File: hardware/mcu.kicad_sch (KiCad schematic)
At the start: 36 parts, among them U1 74LVC125, U2 STM32F407VETx, U3 24LC64, U7 74LVC125, X1 12MHz

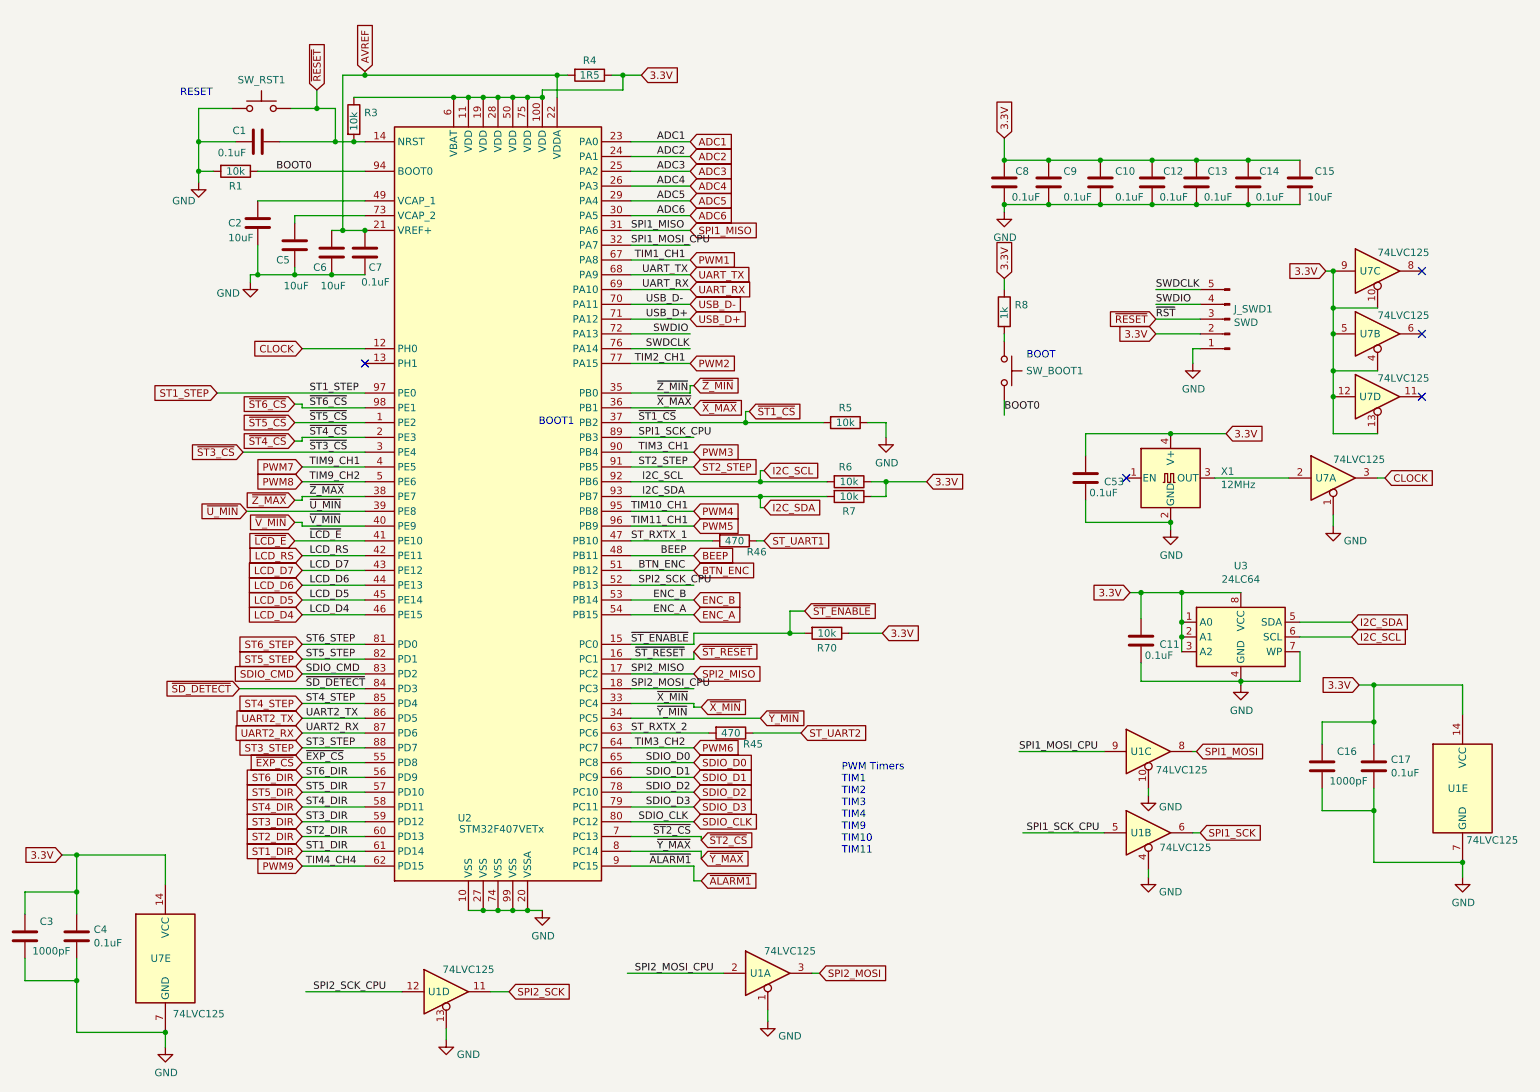
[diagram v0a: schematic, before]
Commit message: Update PrntrBoard fabrication files.
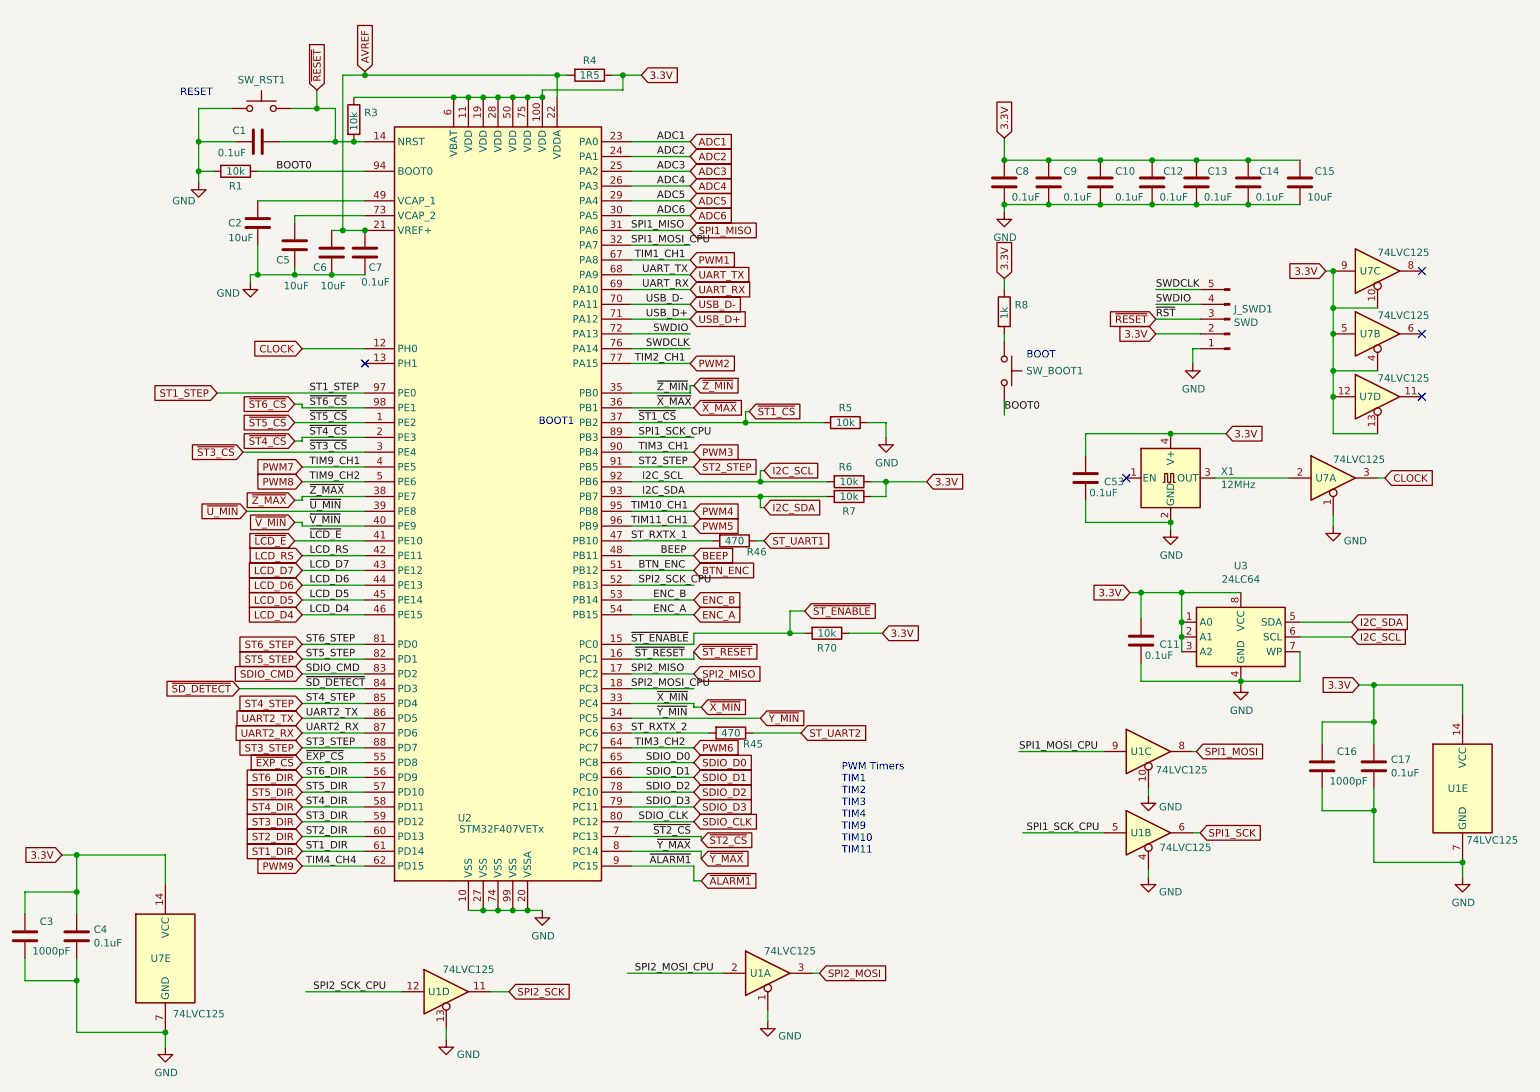
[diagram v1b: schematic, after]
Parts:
- X1: Part # (none) -> SIT1602AI-22-33E-12.000000D; Part# SIT1602AI-22-33E-12.000000D -> (none)
